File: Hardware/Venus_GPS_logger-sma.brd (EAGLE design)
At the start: 31.8 x 19.1 mm, 24 parts, among them U1 VENUS634SMD, U2 33nH, U3 V_REG_LDOSMD, U4 SPI_FLASH-X25XXSMD1

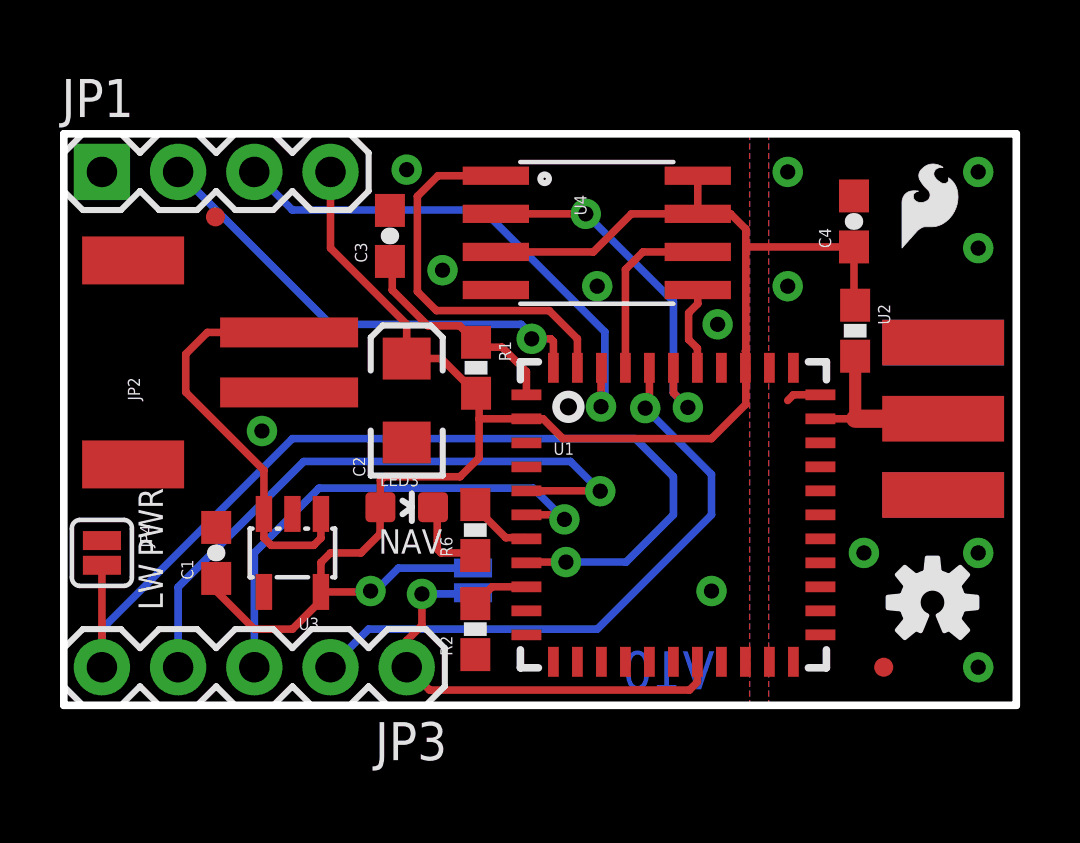
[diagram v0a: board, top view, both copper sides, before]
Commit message: Closed jumper
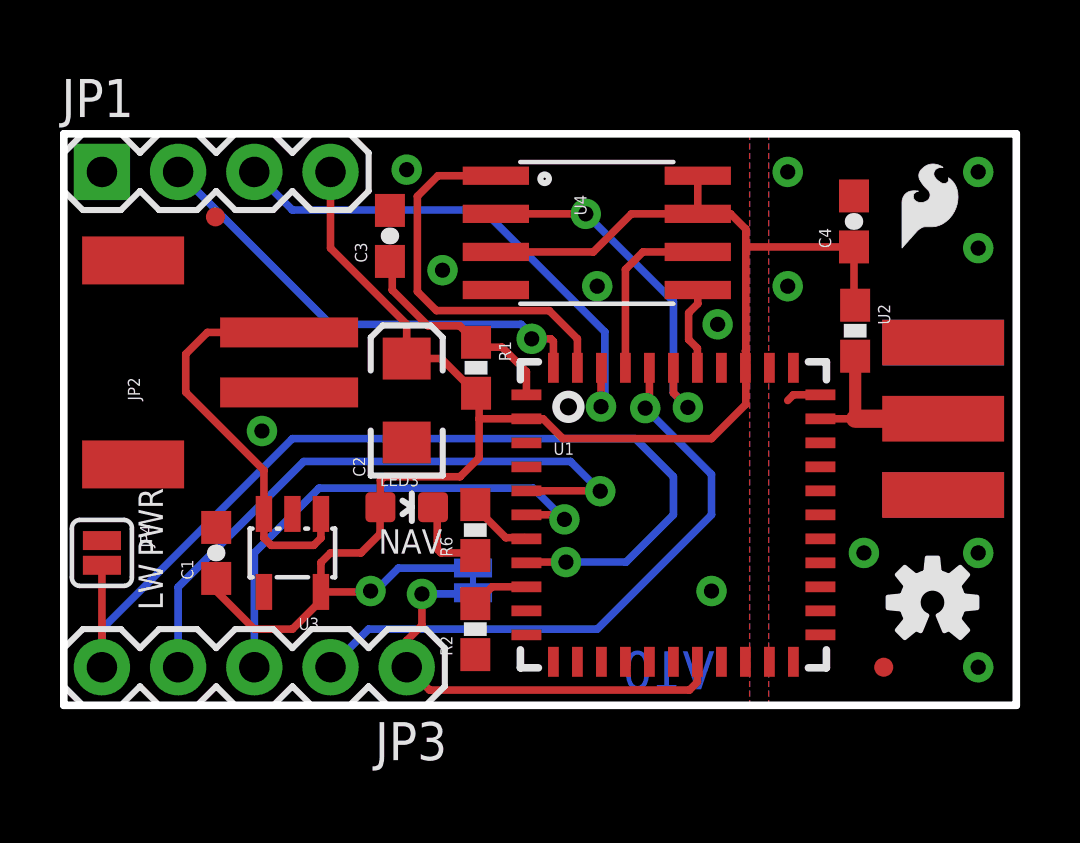
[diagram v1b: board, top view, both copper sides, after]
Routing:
- net N$4: track 0.00 -> 0.69 mm
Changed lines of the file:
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@@
 <setting verticaltext="up"/>
 </settings>
-<grid distance="0.05" unitdist="inch" unit="inch" style="lines" multiple="1" display="yes" altdistance="0.005" altunitdist="inch" altunit="inch"/>
+<grid distance="0.05" unitdist="inch" unit="inch" style="lines" multiple="1" display="yes" altdistance="0.001" altunitdist="inch" altunit="inch"/>
 <layers>
 <layer number="1" name="Top" color="4" fill="1" visible="yes" active="yes"/>
@@
 <layer number="47" name="Measures" color="7" fill="1" visible="no" active="yes"/>
 <layer number="48" name="Document" color="7" fill="1" visible="no" active="yes"/>
-<layer number="49" name="Reference" color="7" fill="1" visible="no" active="yes"/>
+<layer number="49" name="Reference" color="7" fill="1" visible="yes" active="yes"/>
 <layer number="50" name="dxf" color="7" fill="1" visible="no" active="yes"/>
 <layer number="51" name="tDocu" color="6" fill="1" visible="yes" active="yes"/>
@@
 <wire x1="13.6" y1="3.7139" x2="13.6398" y2="3.7537" width="0.254" layer="16"/>
 </signal>
+<signal name="N$2">
+<wire x1="13.589" y1="4.318" x2="13.589" y2="3.937" width="0" layer="19" extent="1-16"/>
+</signal>
+<signal name="N$4">
+<wire x1="13.6398" y1="4.5466" x2="13.6398" y2="3.8608" width="0.2032" layer="16"/>
+</signal>
 </signals>
